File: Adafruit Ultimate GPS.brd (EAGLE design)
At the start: 22.9 x 35.3 mm, 20 parts, among them U1 FGPMMOPA6B, U2 RT9193-3.3

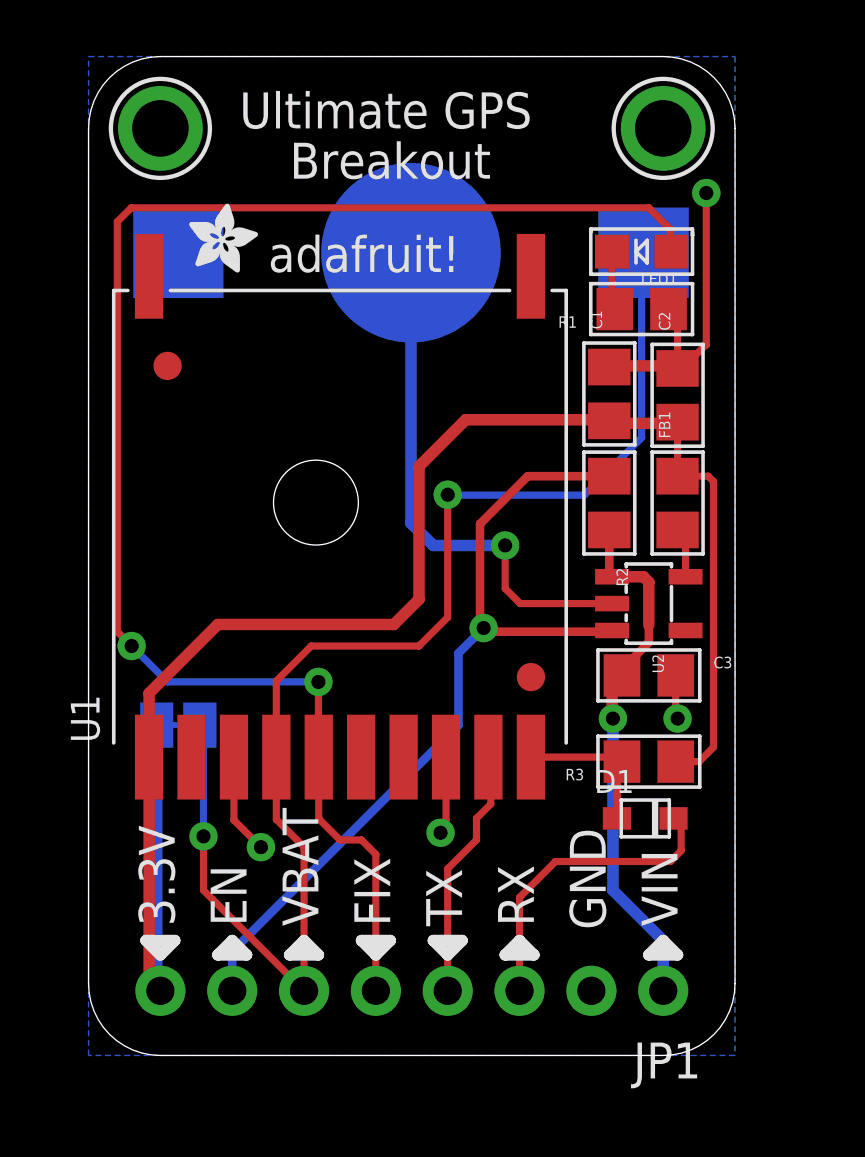
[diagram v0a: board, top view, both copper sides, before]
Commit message: v3!
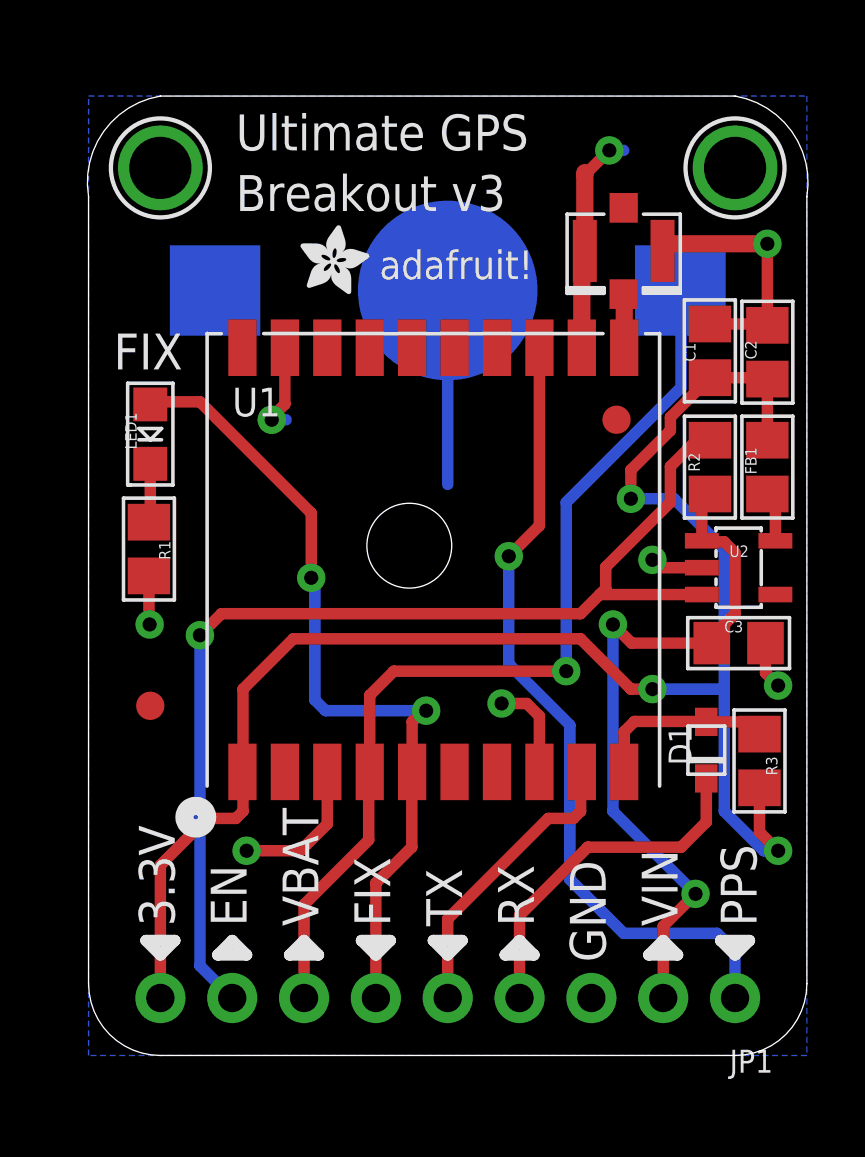
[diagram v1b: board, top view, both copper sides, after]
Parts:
- removed RTC: (no value), microbuilder:SOLDERJUMPER_CLOSEDWIRE
- removed U$16: (no value), microbuilder:ADAFRUIT_TEXT_20MM
- added U$20: U.FL, microbuilder:U.FL
- JP1: device microbuilder:1X08_ROUND_70 -> microbuilder:1X09_ROUND_70
- U1: value FGPMMOPA6B -> FGPMMOPA6H; device microbuilder:FGPMMOPA6B -> microbuilder:FGPMMOPA6H
- moved R1 19.4 mm to (2.13, 17.9), turned to 90 degrees
- moved LED1 18.5 mm to (2.18, 22.0), turned to 180 degrees
- moved FID1 16.0 mm to (18.7, 22.5)
- moved FID2 13.5 mm to (2.18, 12.4)
- moved U$15 4.01 mm to (7.49, 26.9)
- moved R3 3.91 mm to (23.7, 10.4), turned to 90 degrees
- moved C1 3.87 mm to (22.0, 24.9)
- moved R2 3.78 mm to (22.0, 20.8)
- moved U1 3.64 mm to (12.2, 17.5)
- moved C2 3.52 mm to (24.0, 24.9)
- moved FB1 3.42 mm to (24.0, 20.8)
- moved U2 3.42 mm to (23.0, 17.2)
- moved C3 3.37 mm to (23.0, 14.6)
- moved D1 3.24 mm to (21.8, 10.8), turned to 270 degrees
- moved U$9 2.90 mm to (22.9, 31.4)
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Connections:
- new net 1PPS: JP1.1, U1.P$13
- new net N$4: U$20.P$3, U1.P$11
- net 3.3V: now also JP1.9; no longer JP1.8, RTC.2
- net ENABLE: now also JP1.8; no longer JP1.7
- net FIX: now also JP1.6; no longer JP1.5
- net GND: now also JP1.3, U$20.P$1, U$20.P$2, U1.P$12, U1.P$19; no longer JP1.2
- net RX_5V: now also JP1.4; no longer JP1.3
- net TX: now also JP1.5; no longer JP1.4
- net VBACKUP: now also JP1.7; no longer JP1.6, RTC.1
- net VIN: now also JP1.2; no longer JP1.1
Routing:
- net 1PPS: track 0.00 -> 28.7 mm, vias 0 -> 1
- net FIX: track 55.4 -> 29.1 mm
- net VBACKUP: track 48.2 -> 34.1 mm, vias 2 -> 1
- net ENABLE: track 30.4 -> 39.0 mm
- net VIN: track 19.0 -> 25.3 mm, vias 1 -> 2
- net GND: track 38.3 -> 43.1 mm, vias 5 -> 8
- net N$4: track 0.00 -> 1.90 mm
- net TX: track 8.93 -> 10.5 mm
- net 3.3V: track 60.6 -> 59.2 mm, vias 0 -> 3
- net RX_5V: track 11.2 -> 12.4 mm
- net RX: track 5.36 -> 6.54 mm
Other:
- board size 22.9 x 35.3 mm -> 25.5 x 33.9 mm
- board text added: "Breakout v3"
- board text added: "PPS"
- board text removed: "Breakout"
- board text removed: "Cut RTC to"
- board text removed: "RTC"
- board text removed: "enable CR1220"
